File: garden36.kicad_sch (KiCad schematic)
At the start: 82 parts, among them J1 Conn_01x02, J2 Conn_01x02, SW1 SW_SPDT, SW2 SW_Push, SW3 SW_SPDT, SW4 SW_Push, U1 nice_nano, U2 nice_nano

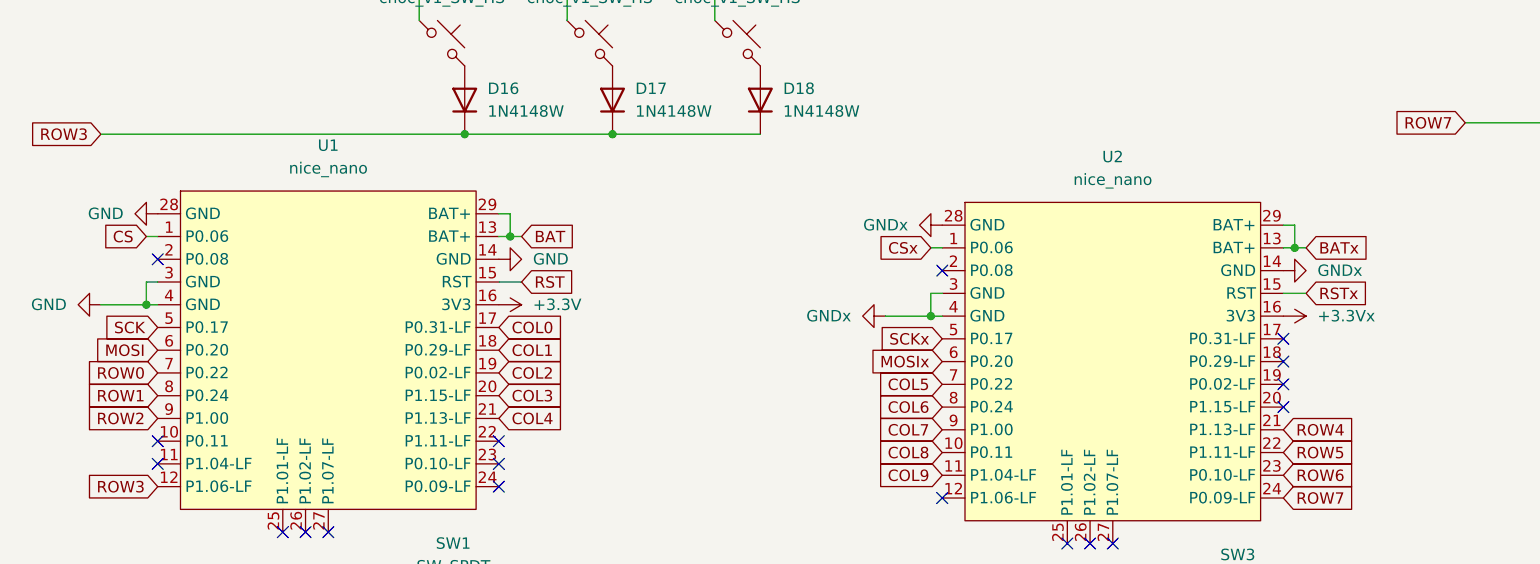
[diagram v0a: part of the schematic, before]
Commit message: V1 ordered
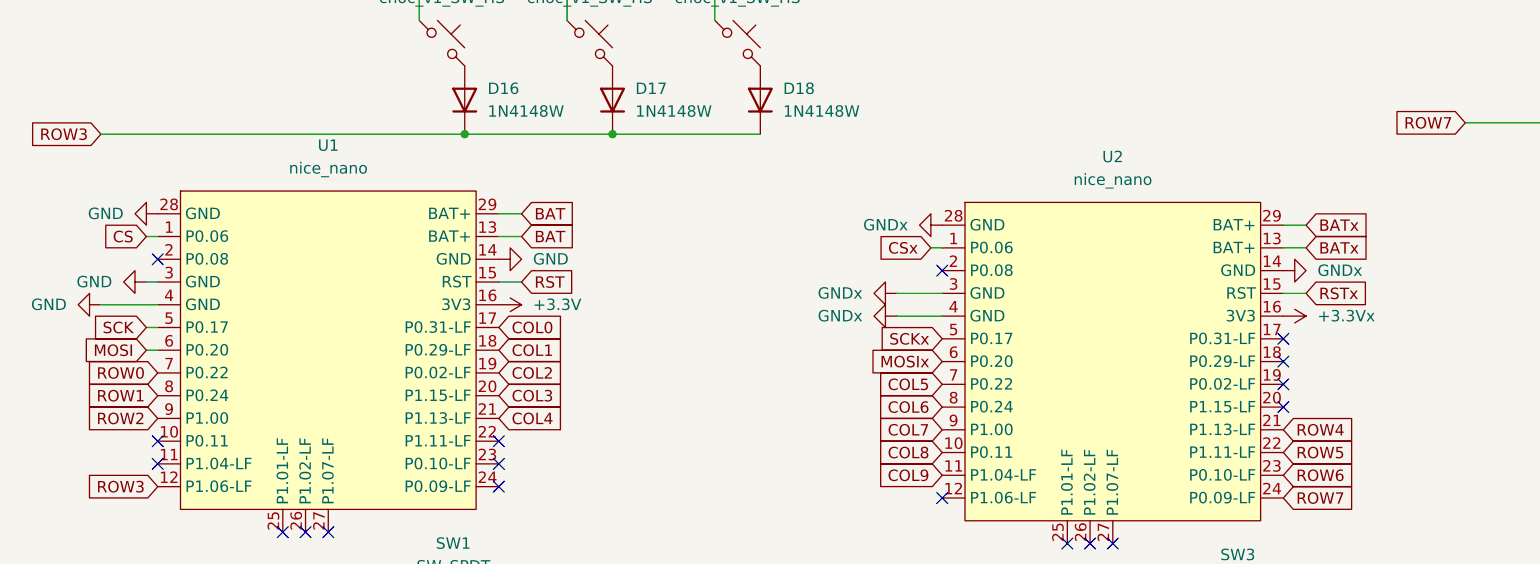
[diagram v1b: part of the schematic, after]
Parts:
- J1, J2: footprint PCM_marbastlib-various:CON_JST_ACH_BM02B -> Connector_JST:JST_PH_S2B-PH-K_1x02_P2.00mm_Horizontal

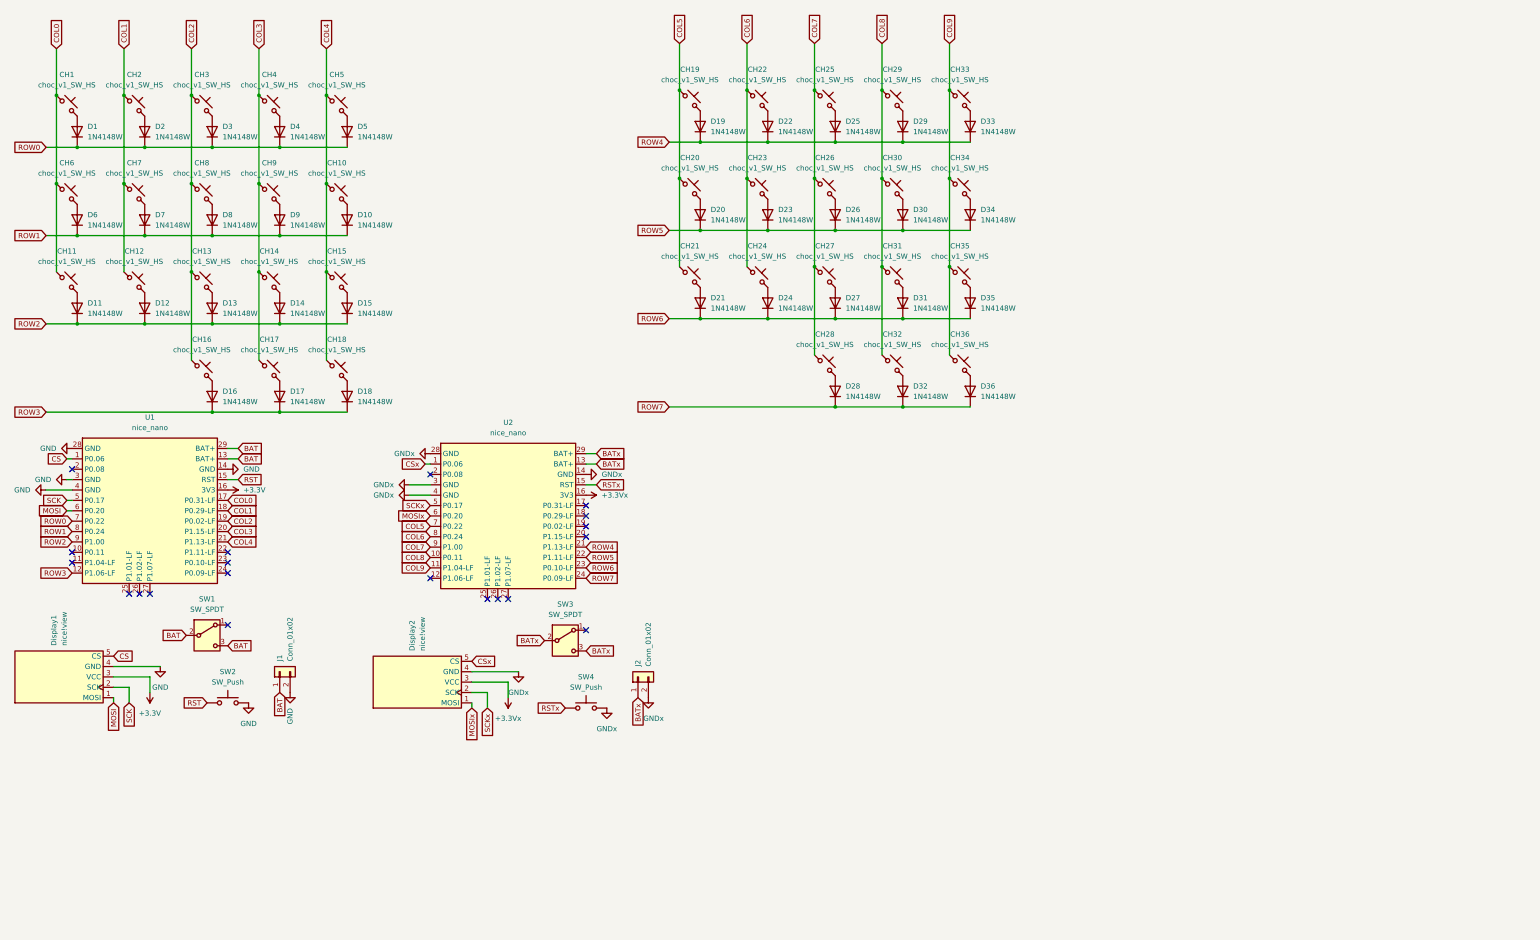
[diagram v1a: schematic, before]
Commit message: V2 started
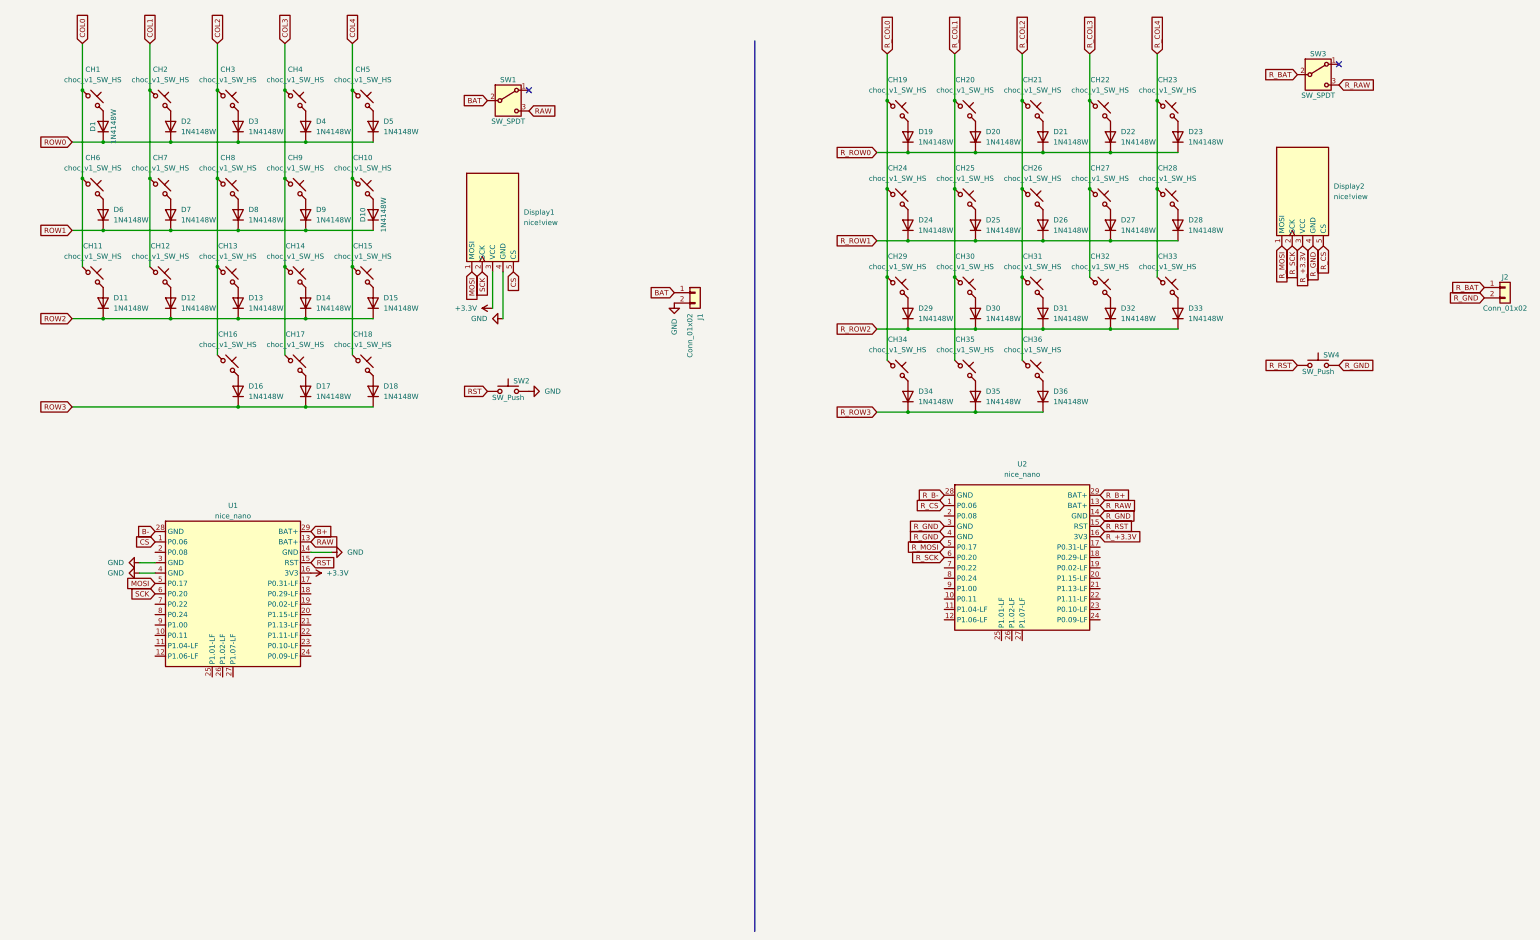
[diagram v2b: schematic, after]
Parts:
- U1, U2: now left out of the parts list
- renumbered CH22 to CH20, CH25 to CH21, CH29 to CH22, CH33 to CH23, CH20 to CH24, CH23 to CH25, CH30 to CH27, CH34 to CH28, CH21 to CH29, CH24 to CH30, CH27 to CH31, CH31 to CH32, CH35 to CH33, CH28 to CH34, CH32 to CH35, D22 to D20, D25 to D21, D29 to D22, D33 to D23, D20 to D24, D23 to D25, D30 to D27, D34 to D28, D21 to D29, D24 to D30, D27 to D31, D31 to D32, D35 to D33, D28 to D34, D32 to D35
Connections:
- net BAT: no longer SW1.3 (C), U1.13 (BAT+), U1.29 (BAT+)
- net COL0: no longer U1.17 (P0.31-LF)
- net COL1: no longer U1.18 (P0.29-LF)
- net COL2: no longer U1.19 (P0.02-LF)
- net COL3: no longer U1.20 (P1.15-LF)
- net COL4: no longer U1.21 (P1.13-LF)
- net GND: no longer U1.28 (GND)
- net MOSI: now also U1.5 (P0.17); no longer U1.6 (P0.20)
- net ROW0: no longer U1.7 (P0.22)
- net ROW1: no longer U1.8 (P0.24)
- net ROW2: no longer U1.9 (P1.00)
- net ROW3: no longer U1.12 (P1.06-LF)
- net SCK: now also U1.6 (P0.20); no longer U1.5 (P0.17)
- net +3.3Vx renamed R_+3.3V
- removed net BATx: J2.1 (Pin_1), SW3.2 (B), SW3.3 (C), U2.13 (BAT+), U2.29 (BAT+)
- net COL5 renamed R_COL0
- net R_COL0: now also CH34.1; no longer U2.7 (P0.22)
- net COL6 renamed R_COL1
- net R_COL1: now also CH35.1; no longer U2.8 (P0.24)
- net COL7 renamed R_COL2
- net R_COL2: now also CH36.1; no longer CH34.1, U2.9 (P1.00)
- net COL8 renamed R_COL3
- net R_COL3: no longer CH35.1, U2.10 (P0.11)
- net COL9 renamed R_COL4
- net R_COL4: no longer CH36.1, U2.11 (P1.04-LF)
- net CSx renamed R_CS
- net GNDx renamed R_GND
- net R_GND: no longer U2.28 (GND)
- net MOSIx renamed R_MOSI
- net R_MOSI: now also U2.5 (P0.17); no longer U2.6 (P0.20)
- net ROW4 renamed R_ROW0
- net R_ROW0: no longer U2.21 (P1.13-LF)
- net ROW5 renamed R_ROW1
- net R_ROW1: no longer U2.22 (P1.11-LF)
- net ROW6 renamed R_ROW2
- net R_ROW2: no longer U2.23 (P0.10-LF)
- net ROW7 renamed R_ROW3
- net R_ROW3: no longer U2.24 (P0.09-LF)
- net RSTx renamed R_RST
- net SCKx renamed R_SCK
- net R_SCK: now also U2.6 (P0.20); no longer U2.5 (P0.17)
- new net B+: U1.29 (BAT+)
- new net B-: U1.28 (GND)
- new net RAW: SW1.3 (C), U1.13 (BAT+)
- new net R_B+: U2.29 (BAT+)
- new net R_B-: U2.28 (GND)
- new net R_BAT: J2.1 (Pin_1), SW3.2 (B)
- new net R_RAW: SW3.3 (C), U2.13 (BAT+)
- no-connect marks 20 -> 2
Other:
- moved on the sheet: CH1, CH10, CH11, CH12, CH13, CH14, CH15, CH16, CH17, CH18, CH19, CH2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
